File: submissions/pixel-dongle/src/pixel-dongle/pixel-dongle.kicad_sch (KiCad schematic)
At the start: 38 parts, among them J1 Conn_01x04_MountingPin, J2 USB_A, J3 Conn_01x02_Pin, SW1 SW_Push, SW2 SW_Push, SW3 SW_Push, U1 XIAO-ESP32-C3-DIP

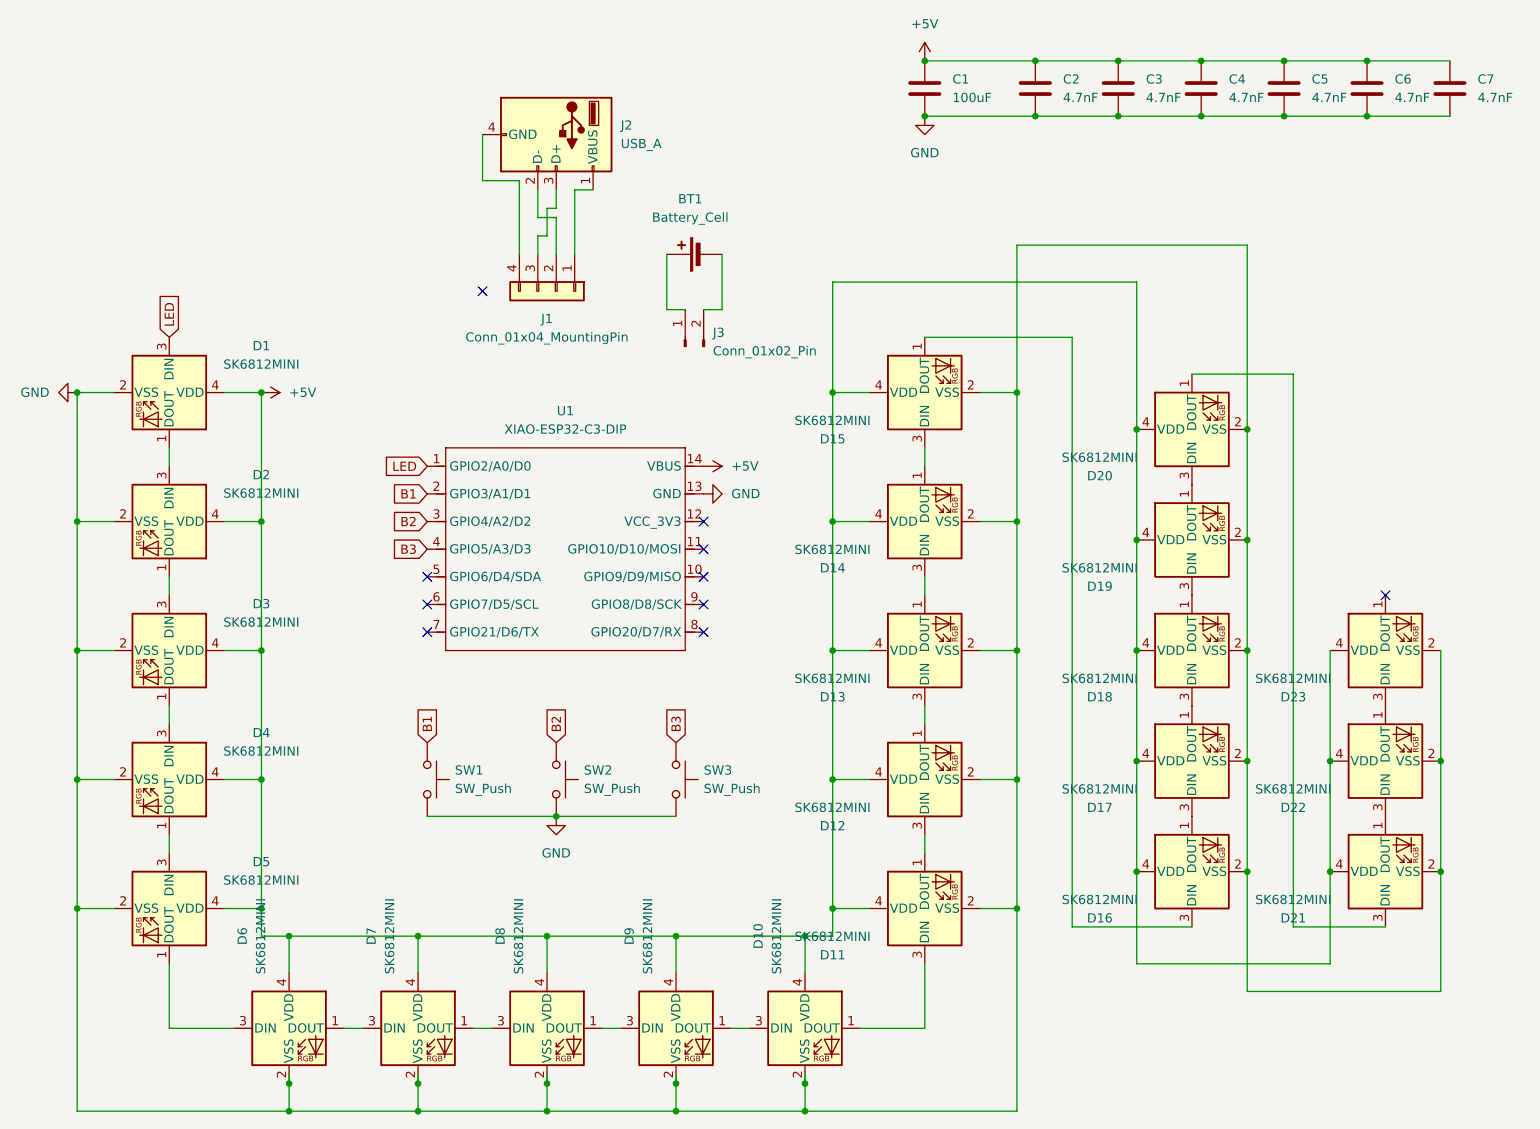
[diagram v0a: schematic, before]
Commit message: updated pixel-dongle and added gerbers (person20020)
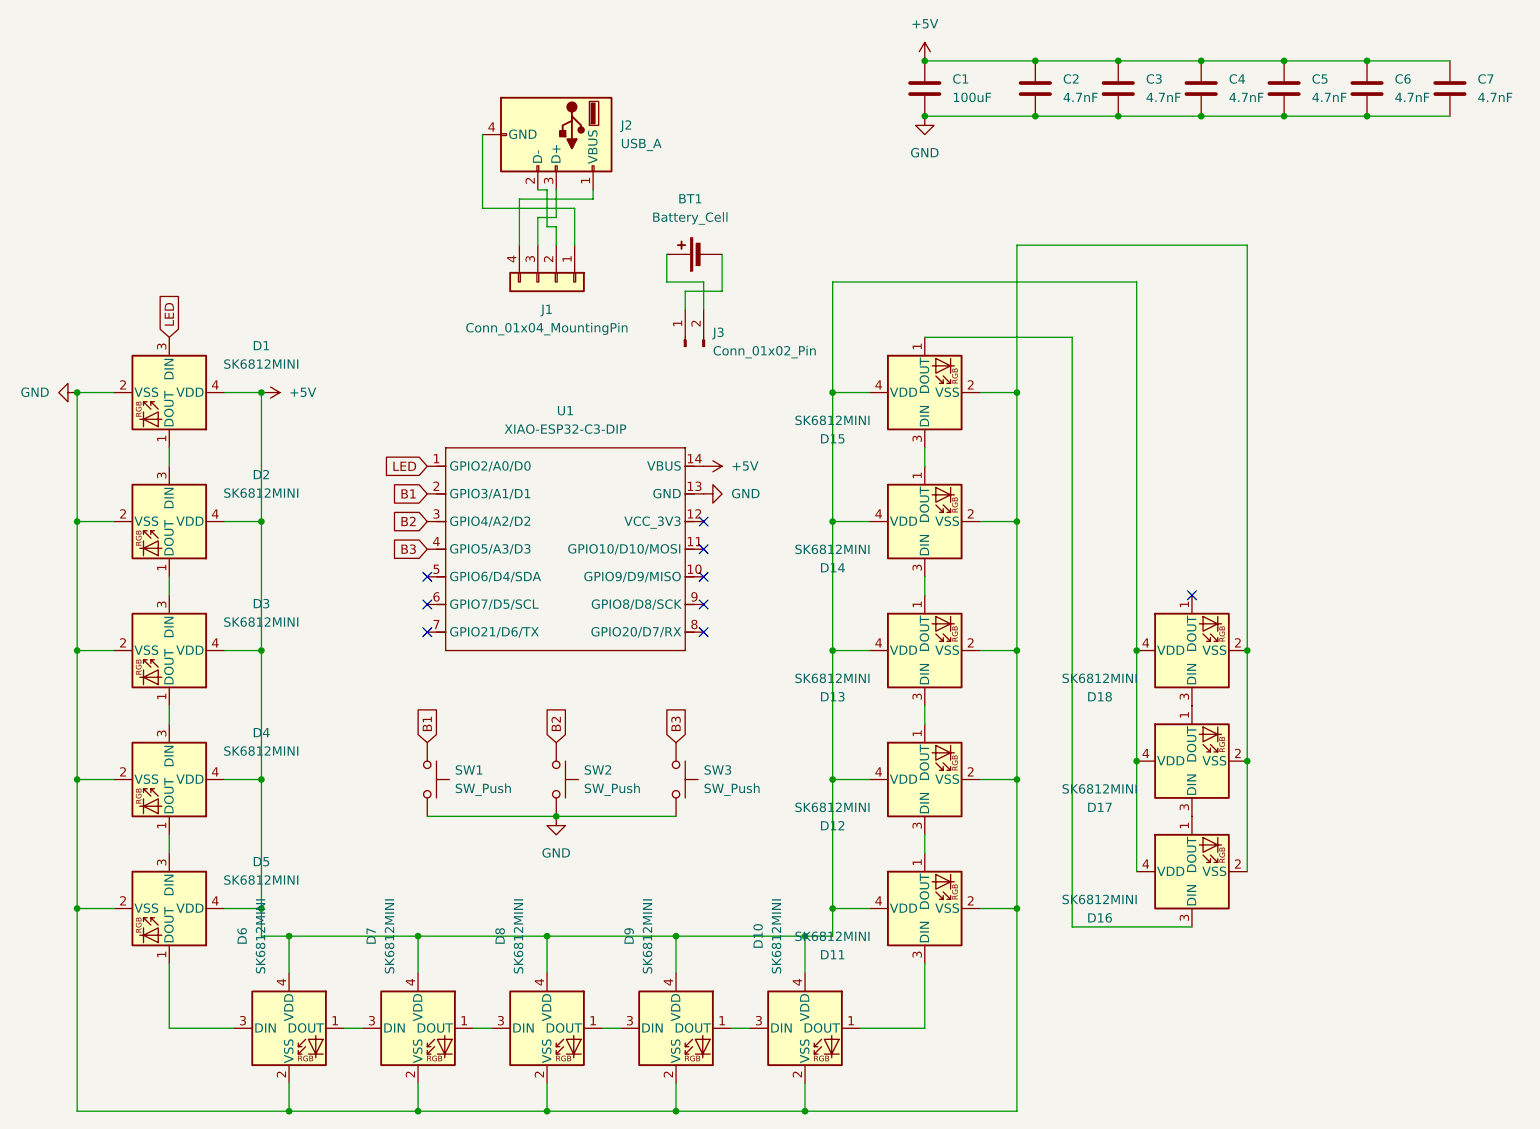
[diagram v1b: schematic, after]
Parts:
- removed D19, D20, D21, D22, D23: SK6812MINI, LED_SMD:LED_SK6812MINI_PLCC4_3.5x3.5mm_P1.75mm, symbol LED:SK6812MINI
- D1, D10, D11, D12, D13, D14, D15, D16, D17, D18, D2, D3, D4, D5, D6, D7, D8, D9: footprint LED_SMD:LED_SK6812MINI_PLCC4_3.5x3.5mm_P1.75mm -> ScottoKeebs_Components:LED_SK6812MINI
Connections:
- net at J2.1 (VBUS): now also J1.4 (Pin_4); no longer J1.1 (Pin_1)
- net at J2.4 (GND): now also J1.1 (Pin_1); no longer J1.4 (Pin_4)
- net at BT1.1 (+): now also J3.2 (Pin_2); no longer J3.1 (Pin_1)
- net at BT1.2 (-): now also J3.1 (Pin_1); no longer J3.2 (Pin_2)
- no-connect marks 10 -> 9
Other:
- title: (none) -> Pixel Dongle
- moved on the sheet: J1
